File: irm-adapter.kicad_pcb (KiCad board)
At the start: 2 copper layers, 82 x 40 mm, 11 parts, among them J1 L, J2 Vout, J3 N, J4 Conn_01x04_Male, J5 Conn_01x04_Male

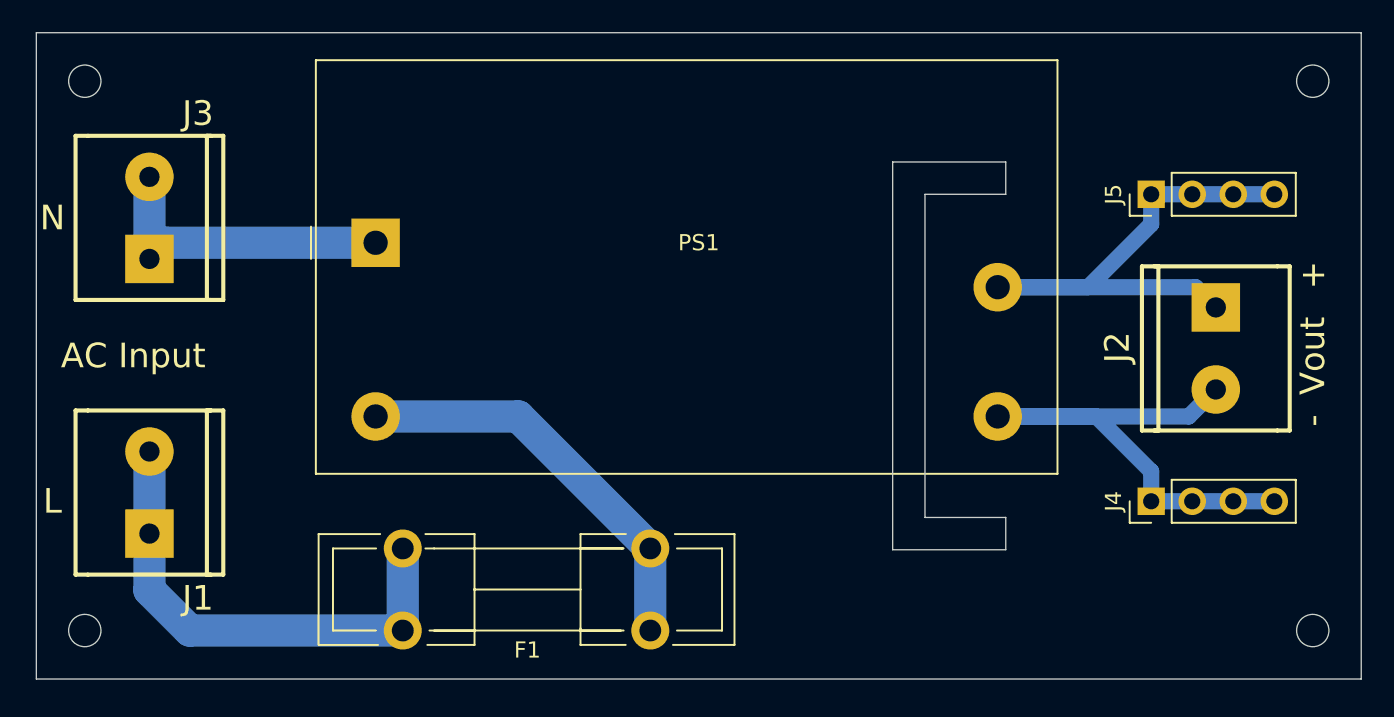
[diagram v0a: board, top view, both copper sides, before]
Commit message: some changes
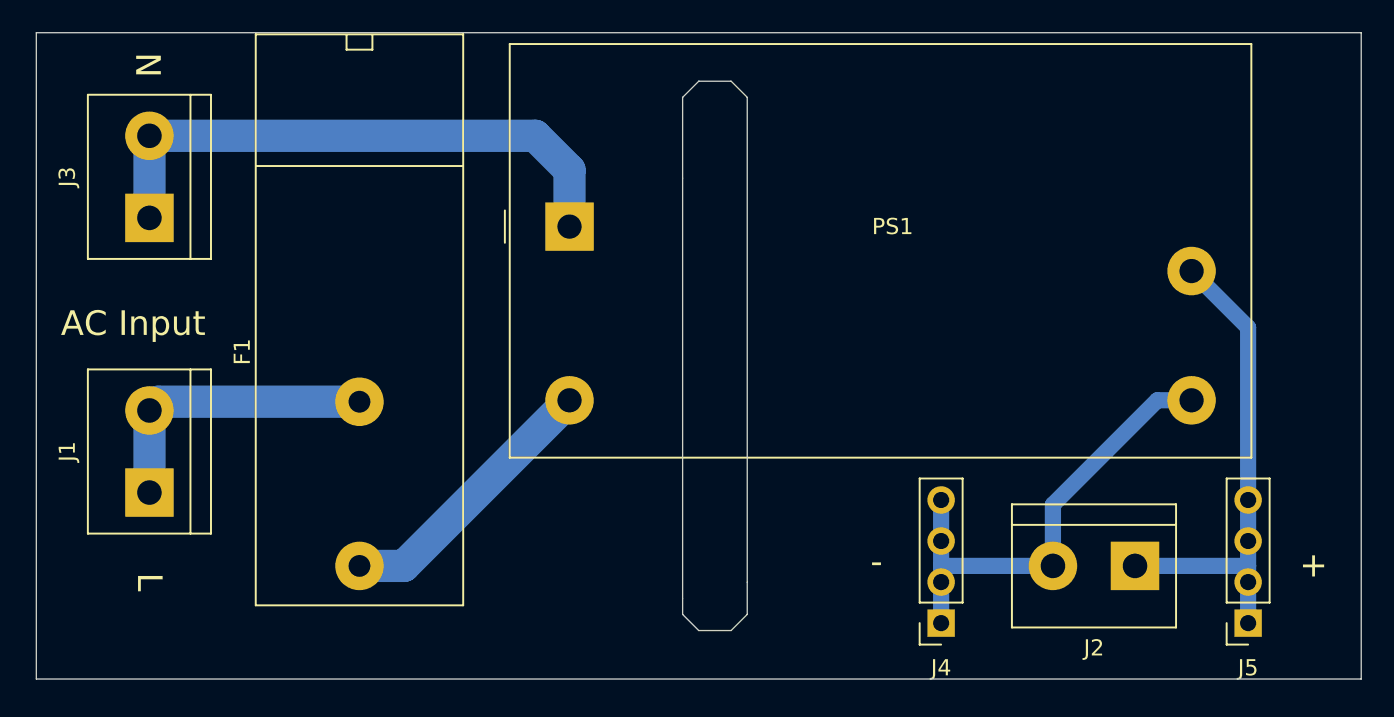
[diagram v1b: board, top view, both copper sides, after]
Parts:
- removed ? (x4): MountingHole_2mm, KiCad Footprints:MountingHole_2mm
- F1: footprint Fuse_Holders_and_Fuses:Fuseholder5x20_horiz_open_lateral_Type-II -> Fuse:Fuseholder_Cylinder-5x20mm_Bulgin_FX0457_Horizontal_Closed
- J1, J2, J3: footprint Screw Terminals:mors_2p -> TerminalBlock:TerminalBlock_bornier-2_P5.08mm
- J4, J5: footprint Pin_Headers:Pin_Header_Straight_1x04_Pitch2.54mm -> Connector_PinSocket_2.54mm:PinSocket_1x04_P2.54mm_Vertical
- PS1: footprint KiCad Footprints:Converter_ACDC_MeanWell_IRM-05-xx_THT -> Converter_ACDC:Converter_ACDC_MeanWell_IRM-05-xx_THT
- moved J5 27.2 mm to (145.0, 76.5), turned to 180 degrees
- moved F1 18.4 mm to (90.0, 73.0), turned to 90 degrees
- moved J4 15.0 mm to (126.0, 76.5), turned to 180 degrees
- moved J2 14.4 mm to (138.0, 73.0), turned to 180 degrees
- moved PS1 12.0 mm to (103.0, 52.0)
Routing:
- net /N: track 19.5 -> 35.5 mm
- net /L: track 30.4 -> 18.3 mm
- net /L_F: track 25.5 -> 17.2 mm
- net /GND: track 34.6 -> 29.6 mm
- net /+5V: track 34.6 -> 30.2 mm
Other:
- outline, holes or cut-outs redrawn
- board text added: "L"
- board text added: "N"
